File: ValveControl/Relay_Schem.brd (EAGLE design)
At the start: 101.6 x 53.6 mm, 69 parts, among them M1 IRLZ44, M2 IRLZ44, M3 IRLZ44, M4 IRLZ44, Q1 LINEAR_REGULATOR, Q2 LINEAR_REGULATOR, Q3 LINEAR_REGULATOR, Q4 LINEAR_REGULATOR, Q5 LINEAR_REGULATOR

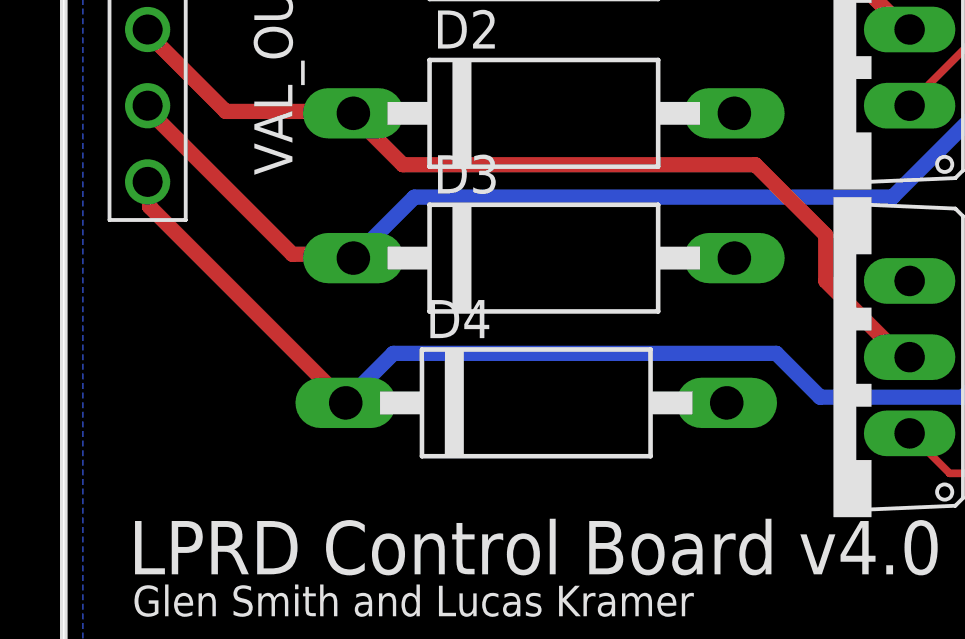
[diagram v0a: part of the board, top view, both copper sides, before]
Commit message: More final tweaks to valve board layout
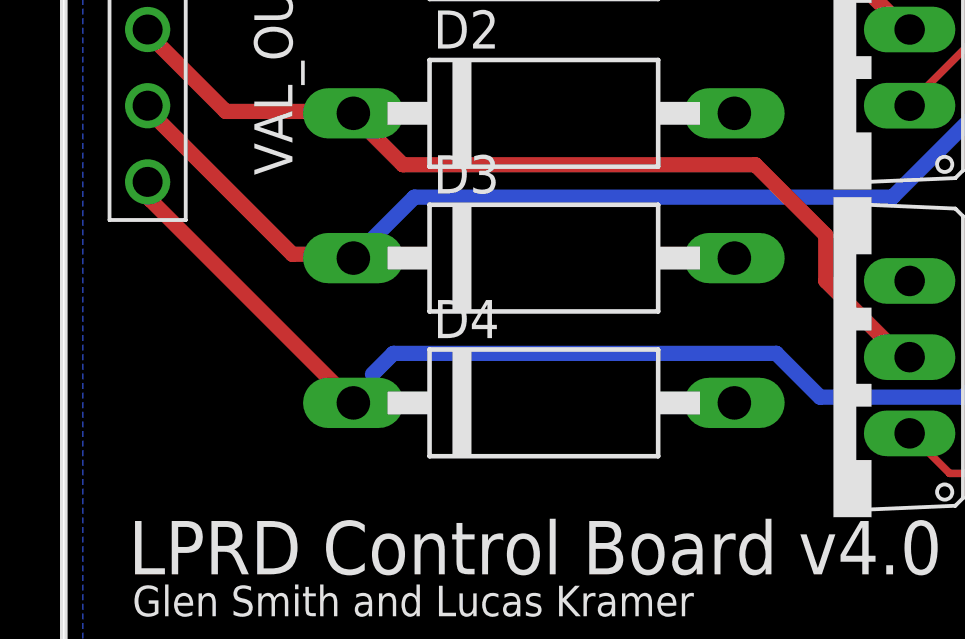
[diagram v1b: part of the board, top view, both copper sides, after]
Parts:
- moved D4 0.25 mm to (16.0, 31.2)
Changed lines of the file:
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@@
 <attribute name="POPULARITY" value="0" x="16.002" y="36.068" size="1.778" layer="27" display="off"/>
 </element>
-<element name="D4" library="diode" library_urn="urn:adsk.eagle:library:210" package="DO15-12" package3d_urn="urn:adsk.eagle:package:43369/2" value="1N5060GP" x="15.748" y="31.242" smashed="yes">
-<attribute name="NAME" x="12.065" y="33.401" size="1.27" layer="25" ratio="10"/>
-<attribute name="POPULARITY" value="0" x="15.748" y="31.242" size="1.778" layer="27" display="off"/>
+<element name="D4" library="diode" library_urn="urn:adsk.eagle:library:210" package="DO15-12" package3d_urn="urn:adsk.eagle:package:43369/2" value="1N5060GP" x="16.002" y="31.242" smashed="yes">
+<attribute name="NAME" x="12.319" y="33.401" size="1.27" layer="25" ratio="10"/>
+<attribute name="POPULARITY" value="0" x="16.002" y="31.242" size="1.778" layer="27" display="off"/>
 </element>
 <element name="MSEL" library="led" library_urn="urn:adsk.eagle:library:259" package="LED3MM" package3d_urn="urn:adsk.eagle:package:15797/1" value="" x="29.845" y="6.985" smashed="yes">
@@
 <element name="M1" library="LPRD_RELAY" package="TO220V" value="IRLZ44" x="25.654" y="43.688" smashed="yes" rot="R90">
 <attribute name="NAME" x="31.6992" y="38.608" size="1.27" layer="25" ratio="10" rot="R90"/>
-<attribute name="VALUE" x="33.274" y="38.608" size="1.27" layer="27" ratio="10" rot="R90"/>
 <attribute name="_EXTERNAL_" value="" x="25.654" y="43.688" size="1.778" layer="27" rot="R90" display="off"/>
 </element>
 <element name="M2" library="LPRD_RELAY" package="TO220V" value="IRLZ44" x="25.654" y="32.766" smashed="yes" rot="R90">
 <attribute name="NAME" x="31.6992" y="27.686" size="1.27" layer="25" ratio="10" rot="R90"/>
-<attribute name="VALUE" x="33.274" y="27.686" size="1.27" layer="27" ratio="10" rot="R90"/>
 <attribute name="_EXTERNAL_" value="" x="25.654" y="32.766" size="1.778" layer="27" rot="R90" display="off"/>
 </element>
 <element name="M3" library="LPRD_RELAY" package="TO220V" value="IRLZ44" x="35.306" y="43.688" smashed="yes" rot="R90">
 <attribute name="NAME" x="41.3512" y="38.608" size="1.27" layer="25" ratio="10" rot="R90"/>
-<attribute name="VALUE" x="42.926" y="38.608" size="1.27" layer="27" ratio="10" rot="R90"/>
 <attribute name="_EXTERNAL_" value="" x="35.306" y="43.688" size="1.778" layer="27" rot="R90" display="off"/>
 </element>
 <element name="M4" library="LPRD_RELAY" package="TO220V" value="IRLZ44" x="35.306" y="32.766" smashed="yes" rot="R90">
 <attribute name="NAME" x="41.3512" y="27.686" size="1.27" layer="25" ratio="10" rot="R90"/>
-<attribute name="VALUE" x="42.926" y="27.686" size="1.27" layer="27" ratio="10" rot="R90"/>
 <attribute name="_EXTERNAL_" value="" x="35.306" y="32.766" size="1.778" layer="27" rot="R90" display="off"/>
 </element>
@@
 <contactref element="VAL_OUT" pad="P$4"/>
 <contactref element="M4" pad="2"/>
-<wire x1="2.8575" y1="37.7825" x2="2.8575" y2="38.4175" width="0.508" layer="1"/>
+<wire x1="2.8575" y1="38.0365" x2="2.8575" y2="38.4175" width="0.508" layer="1"/>
 <wire x1="2.8575" y1="38.4175" x2="2.794" y2="38.608" width="0.254" layer="1"/>
-<wire x1="2.8575" y1="37.7825" x2="9.398" y2="31.242" width="0.508" layer="1"/>
+<wire x1="2.8575" y1="38.0365" x2="9.652" y2="31.242" width="0.508" layer="1"/>
 <wire x1="37.1475" y1="32.0675" x2="37.846" y2="32.766" width="0.508" layer="16"/>
 <wire x1="30.607" y1="32.0675" x2="37.1475" y2="32.0675" width="0.508" layer="16"/>
@@
 <wire x1="23.749" y1="32.893" x2="25.2095" y2="31.4325" width="0.508" layer="16"/>
 <wire x1="10.9855" y1="32.893" x2="23.749" y2="32.893" width="0.508" layer="16"/>
-<wire x1="9.525" y1="31.4325" x2="10.9855" y2="32.893" width="0.508" layer="16"/>
-<wire x1="9.525" y1="31.4325" x2="9.398" y2="31.242" width="0.254" layer="16"/>
+<wire x1="10.287" y1="32.1945" x2="10.9855" y2="32.893" width="0.508" layer="16"/>
+<wire x1="10.287" y1="32.1945" x2="9.652" y2="31.242" width="0.254" layer="16"/>
 </signal>
 <signal name="N$10">
